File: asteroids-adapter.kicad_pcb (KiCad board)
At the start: 2 copper layers, 88 x 90.2 mm, 15 parts, among them J1 Asteroids PCB connector, J2 Asteroids harness connector, U1 TL074

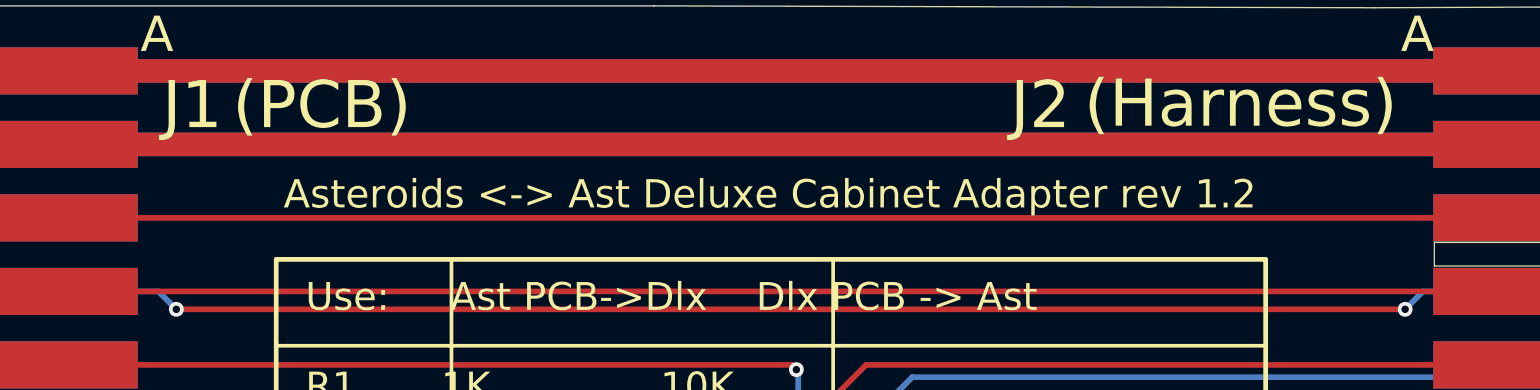
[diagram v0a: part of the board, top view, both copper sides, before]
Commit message: Update to rev 1.3
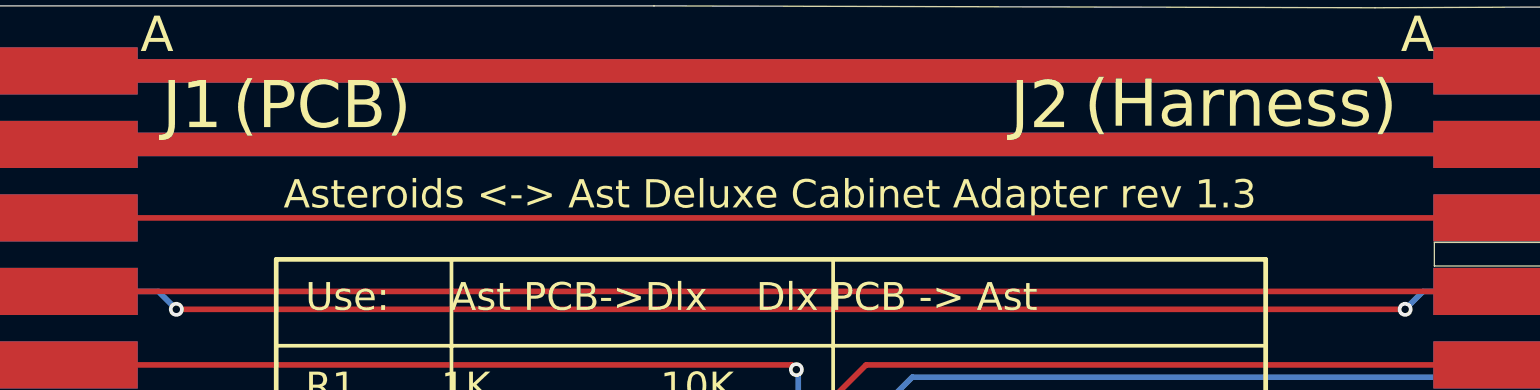
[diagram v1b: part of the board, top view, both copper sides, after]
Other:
- board text added: "Asteroids <-> Ast Deluxe Cabinet Adapter rev 1.3"
- board text removed: "Asteroids <-> Ast Deluxe Cabinet Adapter rev 1.2"
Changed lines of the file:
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@@
   (title_block
     (title "Asteroids to Asteroids Deluxe Adapter")
-    (date "2022-02-22")
-    (rev "1.2")
+    (date "2022-02-24")
+    (rev "1.3")
   )
   (layers
@@
     (effects (font (size 1.905 1.905) (thickness 0.3)) (justify mirror))
   )
-  (gr_text "Asteroids <-> Ast Deluxe Cabinet Adapter rev 1.2" (at 150.5204 62.5856) (layer "F.SilkS")
+  (gr_text "Asteroids <-> Ast Deluxe Cabinet Adapter rev 1.3" (at 150.5204 62.5856) (layer "F.SilkS")
     (effects (font (size 1.524 1.524) (thickness 0.3)))
   )
